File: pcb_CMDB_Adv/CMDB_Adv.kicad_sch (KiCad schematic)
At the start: 1 part, among them J1 POWER TERMINAL

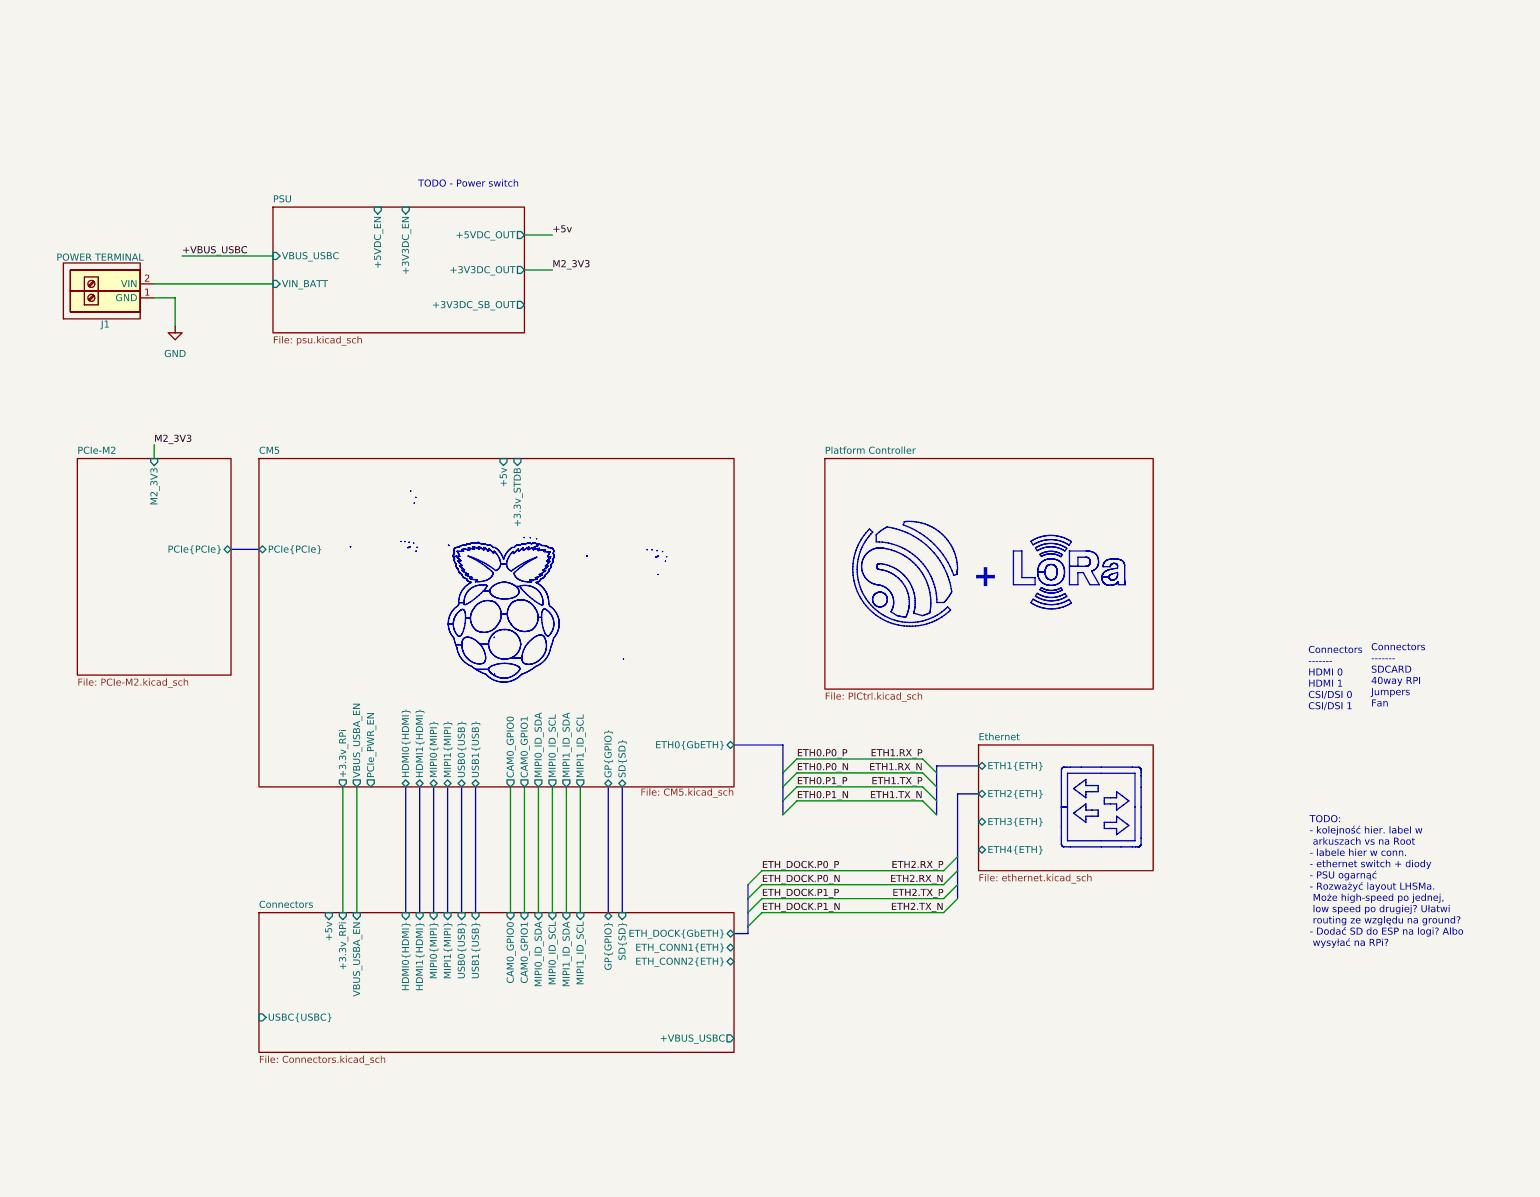
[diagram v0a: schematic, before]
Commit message: CMDB-Adv PCB WIP
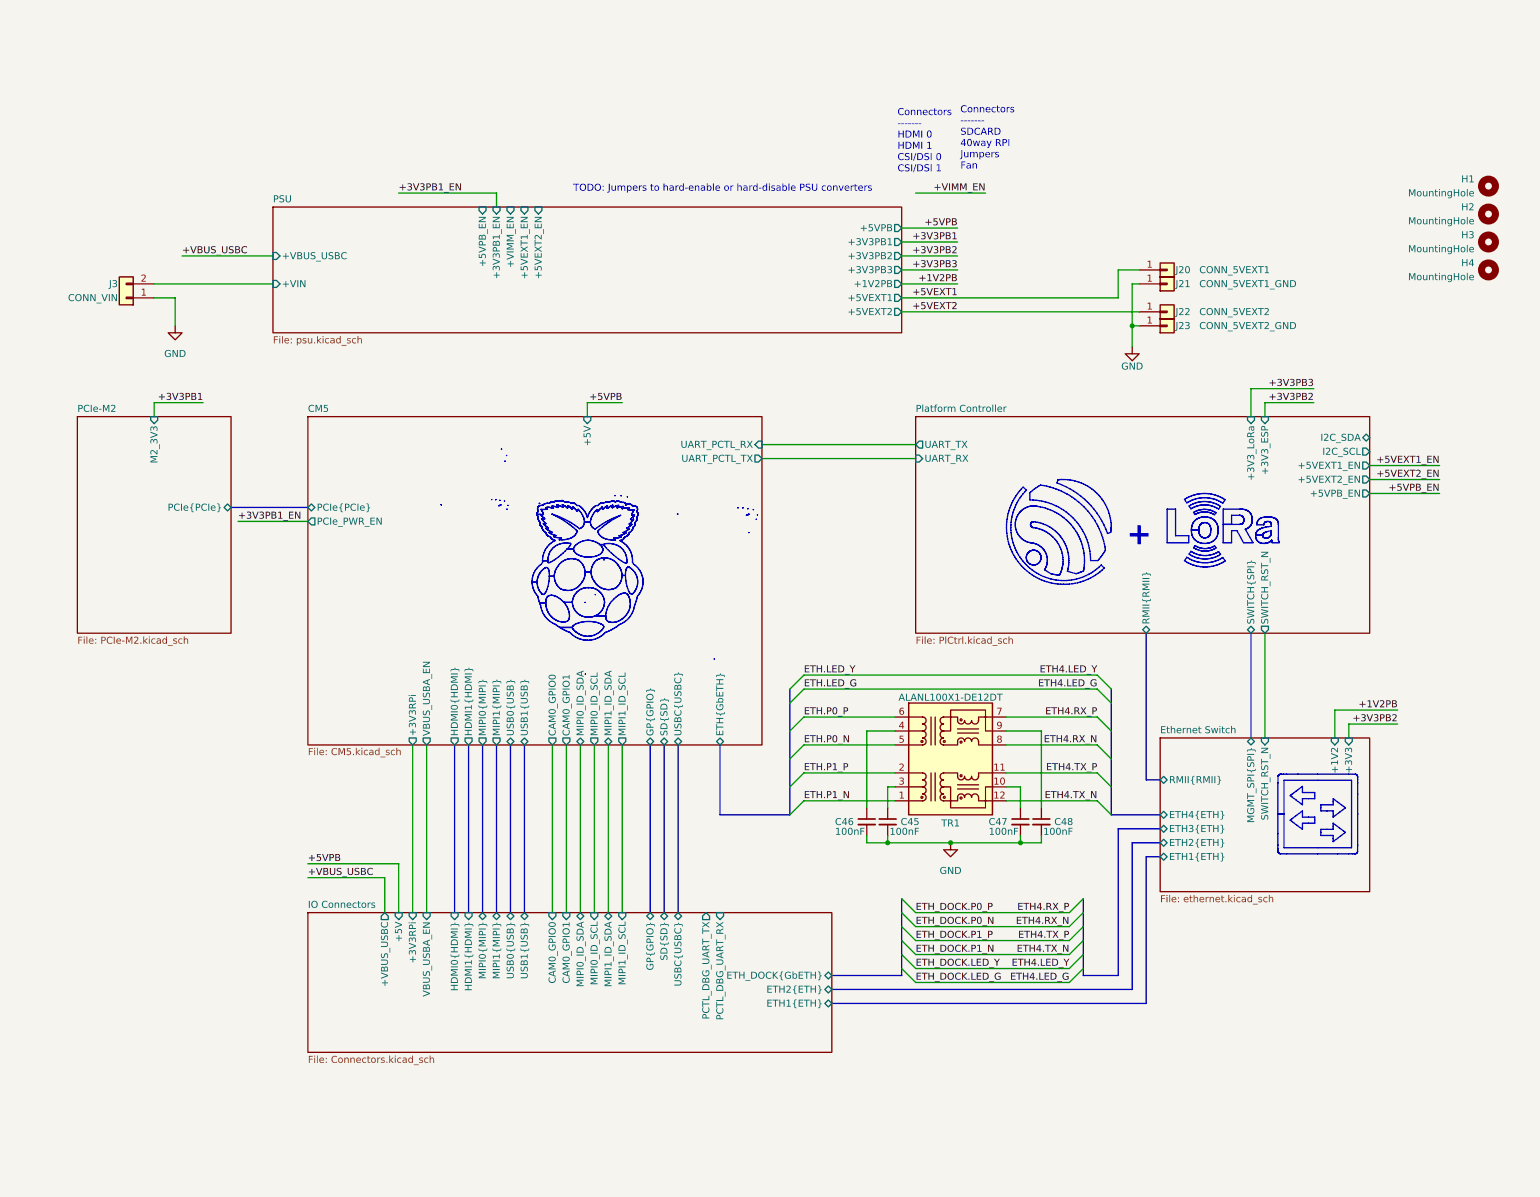
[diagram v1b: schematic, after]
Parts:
- removed J1: POWER TERMINAL, CMDB_Adv:Power Terminal, symbol CMDB_Adv:Power_Terminal
- added C45, C46, C47, C48: 100nF, Capacitor_SMD:C_0402_2012Metric_Pad1.18x1.45mm_HandSolder, symbol Device:C_Small
- added H1, H2, H3, H4: MountingHole, CMDB_Adv:MountingHole_2.7mm_M2.5_DIN965, symbol Mechanical:MountingHole
- added J20: CONN_5VEXT1, Connector_Wire:SolderWirePad_1x01_SMD_3x6mm, symbol Connector_Generic:Conn_01x01
- added J21: CONN_5VEXT1_GND, Connector_Wire:SolderWirePad_1x01_SMD_3x6mm, symbol Connector_Generic:Conn_01x01
- added J22: CONN_5VEXT2, Connector_Wire:SolderWirePad_1x01_SMD_3x6mm, symbol Connector_Generic:Conn_01x01
- added J23: CONN_5VEXT2_GND, Connector_Wire:SolderWirePad_1x01_SMD_3x6mm, symbol Connector_Generic:Conn_01x01
- added J3: CONN_VIN, Connector_AMASS:AMASS_XT30PW-M_1x02_P2.50mm_Horizontal, symbol Connector_Generic:Conn_01x02
- added TR1: ALANL100X1-DE12DT, CMDB_Adv:ALANL100X1DE12DT, symbol CMDB_Adv:ALANL100X1DE12DT
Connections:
- net GND: now also C45.2, C46.2, C47.2, C48.2, J21.1 (Pin_1), J23.1 (Pin_1), J3.1 (Pin_1)
- new net: C48.1, TR1.9 (C_RX)
- new net: C46.1, TR1.4 (C_RD)
- new net: C47.1, TR1.10 (C_TX)
- new net: C45.1, TR1.3 (C_TD)
- new net +5VEXT1: J20.1 (Pin_1)
- new net +5VEXT2: J22.1 (Pin_1)
- new net ETH.P0_N: TR1.5 (RD+)
- new net ETH.P0_P: TR1.6 (RD-)
- new net ETH.P1_N: TR1.1 (TD+)
- new net ETH.P1_P: TR1.2 (TD-)
- new net ETH4.RX_N: TR1.8 (RX+)
- new net ETH4.RX_P: TR1.7 (RX-)
- new net ETH4.TX_N: TR1.12 (TX+)
- new net ETH4.TX_P: TR1.11 (TX-)
- new net PSU/+VIN: J3.2 (Pin_2)
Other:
- sheet Connectors renamed IO Connectors
- sheet Ethernet renamed Ethernet Switch
- sheet CM5 ports: added +3V3RPi, +5V, ETH{GbETH}, UART_PCTL_RX, UART_PCTL_TX, USBC{USBC}; removed +3.3v_RPi, +3.3v_STDB, +5v, ETH0{GbETH}
- sheet Ethernet Switch ports: added +1V2, +3V3, MGMT_SPI{SPI}, RMII{RMII}, SWITCH_RST_N; removed none
- sheet IO Connectors ports: added +3V3RPi, +5V, ETH1{ETH}, ETH2{ETH}, PCTL_DBG_UART_RX, PCTL_DBG_UART_TX; removed +3.3v_RPi, +5v, ETH_CONN1{ETH}, ETH_CONN2{ETH}
- sheet PSU ports: added +1V2PB, +3V3PB1, +3V3PB1_EN, +3V3PB2, +3V3PB3, +5VEXT1, +5VEXT1_EN, +5VEXT2, +5VEXT2_EN, +5VPB, +5VPB_EN, +VBUS_USBC, +VIMM_EN, +VIN; removed +3V3DC_EN, +3V3DC_OUT, +3V3DC_SB_OUT, +5VDC_EN, +5VDC_OUT, VBUS_USBC, VIN_BATT
- sheet Platform Controller ports: added +3V3_ESP, +3V3_LoRa, +5VEXT1_EN, +5VEXT2_EN, +5VPB_EN, I2C_SCL, I2C_SDA, RMII{RMII}, SWITCH_RST_N, SWITCH{SPI}, UART_RX, UART_TX; removed none
- note added: "TODO: Jumpers to hard-enable or hard-disable PSU converters"
- note removed: "TODO - Power switch"
- note removed: "TODO: - kolejność hier. label w arkuszach vs na Root - labele hier w conn. - ethernet switch + diody - PSU ogarnąć - Rozważyć layout LHSMa. Może high-speed po jednej, low speed po drugiej? Ułatwi routing ze względu na ground? - Dodać SD do ESP na logi? Albo wysyłać na RPi?"

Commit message: CMDB_Adv WIP
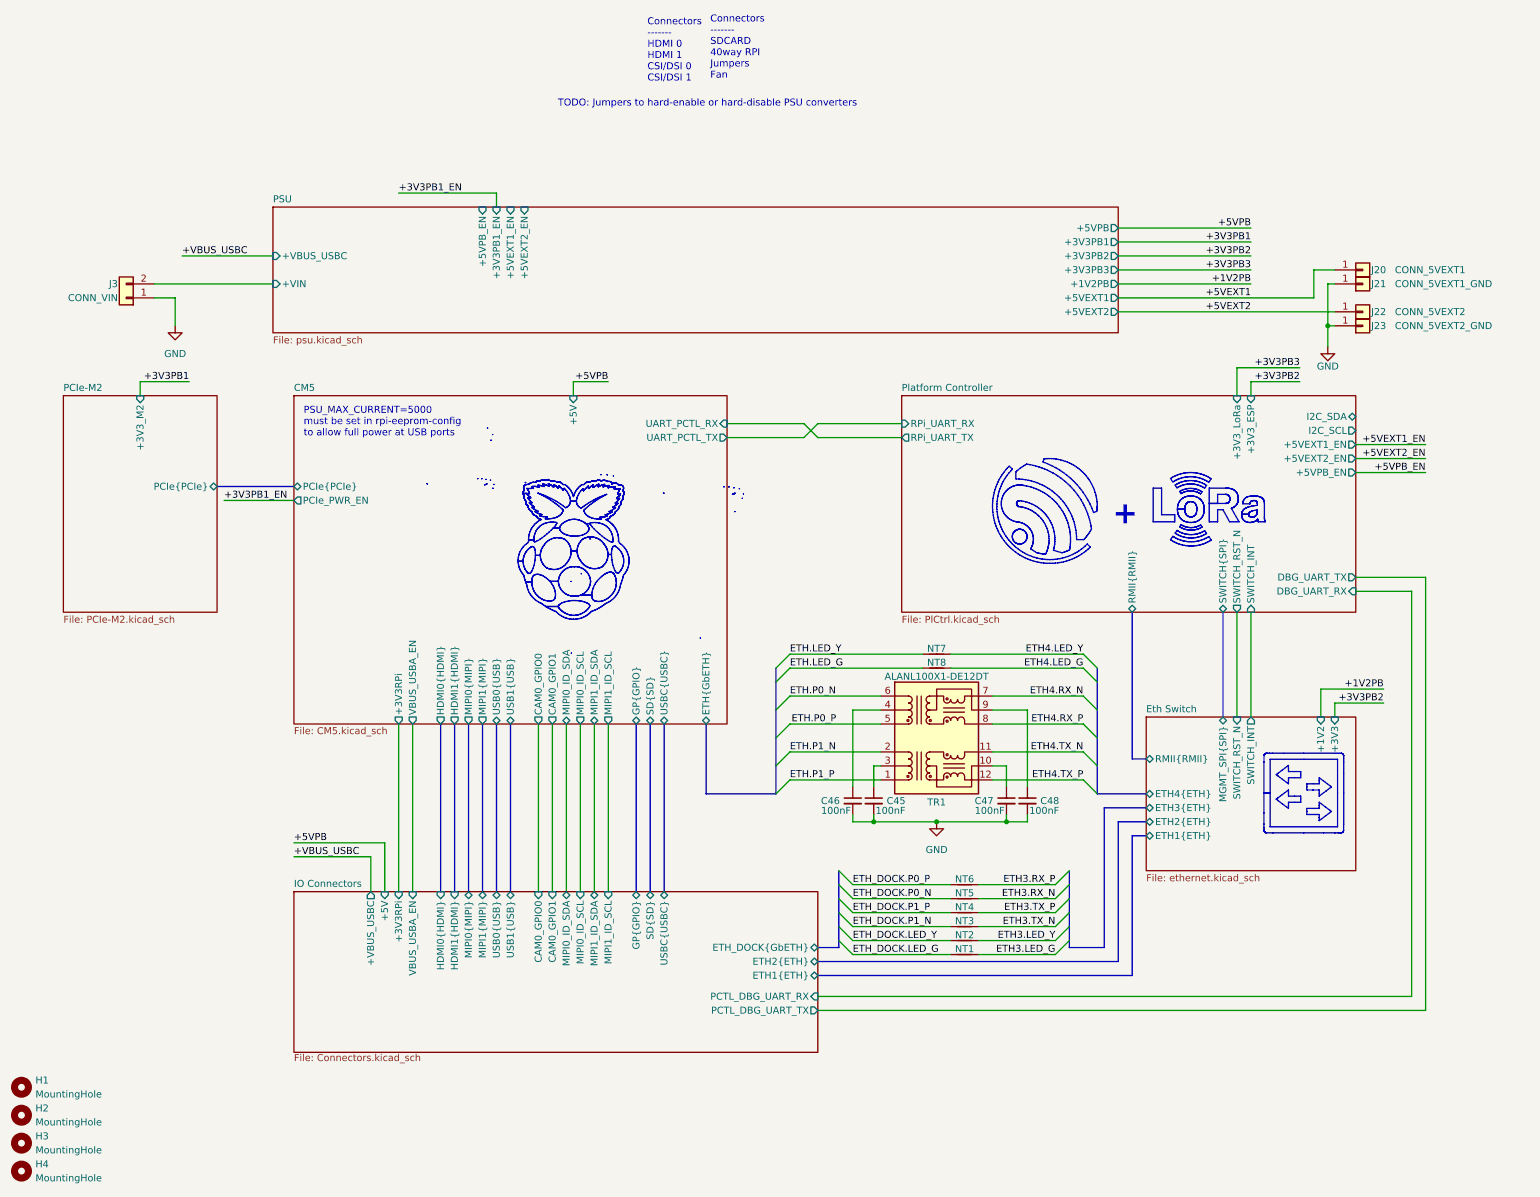
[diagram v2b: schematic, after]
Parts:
- added NT1, NT2, NT3, NT4, NT5, NT6, NT7, NT8: NetTie_2, NetTie:NetTie-2_SMD_Pad0.5mm, symbol Device:NetTie_2
- C45, C46, C47, C48: footprint Capacitor_SMD:C_0402_2012Metric_Pad1.18x1.45mm_HandSolder -> Capacitor_SMD:C_0402_1005Metric_Pad0.74x0.62mm_HandSolder
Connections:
- net ETH.LED_G: now also NT8.1
- net ETH.LED_Y: now also NT7.1
- net ETH.P0_N: now also TR1.6 (RD-); no longer TR1.5 (RD+)
- net ETH.P0_P: now also TR1.5 (RD+); no longer TR1.6 (RD-)
- net ETH.P1_N: now also TR1.2 (TD-); no longer TR1.1 (TD+)
- net ETH.P1_P: now also TR1.1 (TD+); no longer TR1.2 (TD-)
- net ETH4.RX_N: now also TR1.7 (RX-); no longer TR1.8 (RX+)
- net ETH4.RX_P: now also TR1.8 (RX+); no longer TR1.7 (RX-)
- net ETH4.TX_N: now also TR1.11 (TX-); no longer TR1.12 (TX+)
- net ETH4.TX_P: now also TR1.12 (TX+); no longer TR1.11 (TX-)
- new net ETH3.LED_G: NT1.2
- new net ETH3.LED_Y: NT2.2
- new net ETH3.RX_N: NT5.2
- new net ETH3.RX_P: NT6.2
- new net ETH3.TX_N: NT3.2
- new net ETH3.TX_P: NT4.2
- new net ETH4.LED_G: NT8.2
- new net ETH4.LED_Y: NT7.2
- new net ETH_DOCK.LED_G: NT1.1
- new net ETH_DOCK.LED_Y: NT2.1
- new net ETH_DOCK.P0_N: NT5.1
- new net ETH_DOCK.P0_P: NT6.1
- new net ETH_DOCK.P1_N: NT3.1
- new net ETH_DOCK.P1_P: NT4.1
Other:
- sheet Ethernet Switch renamed Eth Switch
- sheet Eth Switch ports: added SWITCH_INT; removed none
- sheet PCIe-M2 ports: added +3V3_M2; removed M2_3V3
- sheet PSU ports: added none; removed +VIMM_EN
- sheet Platform Controller ports: added DBG_UART_RX, DBG_UART_TX, RPi_UART_RX, RPi_UART_TX, SWITCH_INT; removed UART_RX, UART_TX
- note added: "PSU_MAX_CURRENT=5000 must be set in rpi-eeprom-config to allow full power at USB ports"
- moved on the sheet: C45, C46, C47, C48, H1, H2, H3, H4, J20, J21, J22, J23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
